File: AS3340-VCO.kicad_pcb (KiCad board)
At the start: 2 copper layers, 90.9 x 101.6 mm, 61 parts, among them J1 1V/OCT_INPUT, J10 SAWTOOTH_OUT, J11 TRIANGLE_OUT, J2 1V/OCT_OUT, J3 CV2_INPUT, J4 EXT_PWM_CTRL_INPUT, J5 POSITIVE_HARD_SYNC_INPUT, J6 NEGATIVE_HARD_SYNC_INPUT, J7 SOFT_SYNC_INPUT, J8 FM_INPUT, J9 SQUARE_OUT, SW1 SW_SPDT, U1 TL074, U2 AS3340

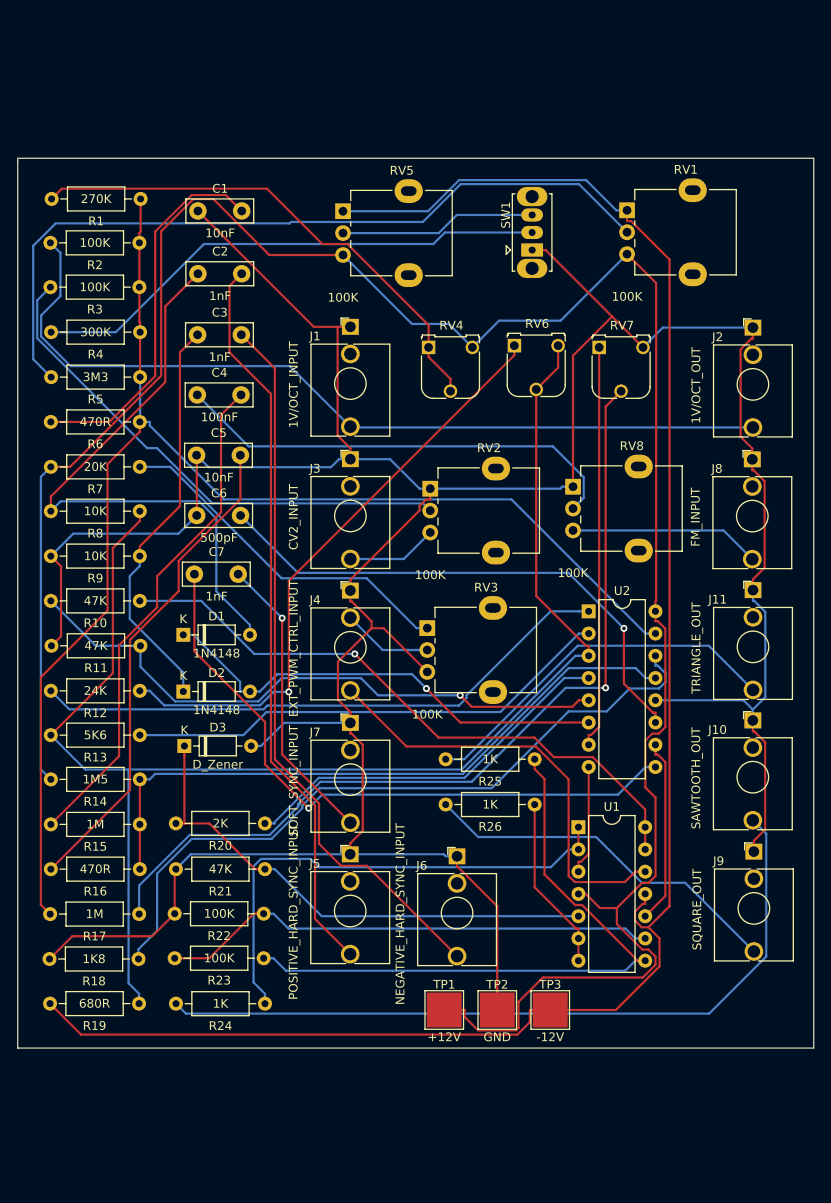
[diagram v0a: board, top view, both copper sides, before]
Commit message: Refactor
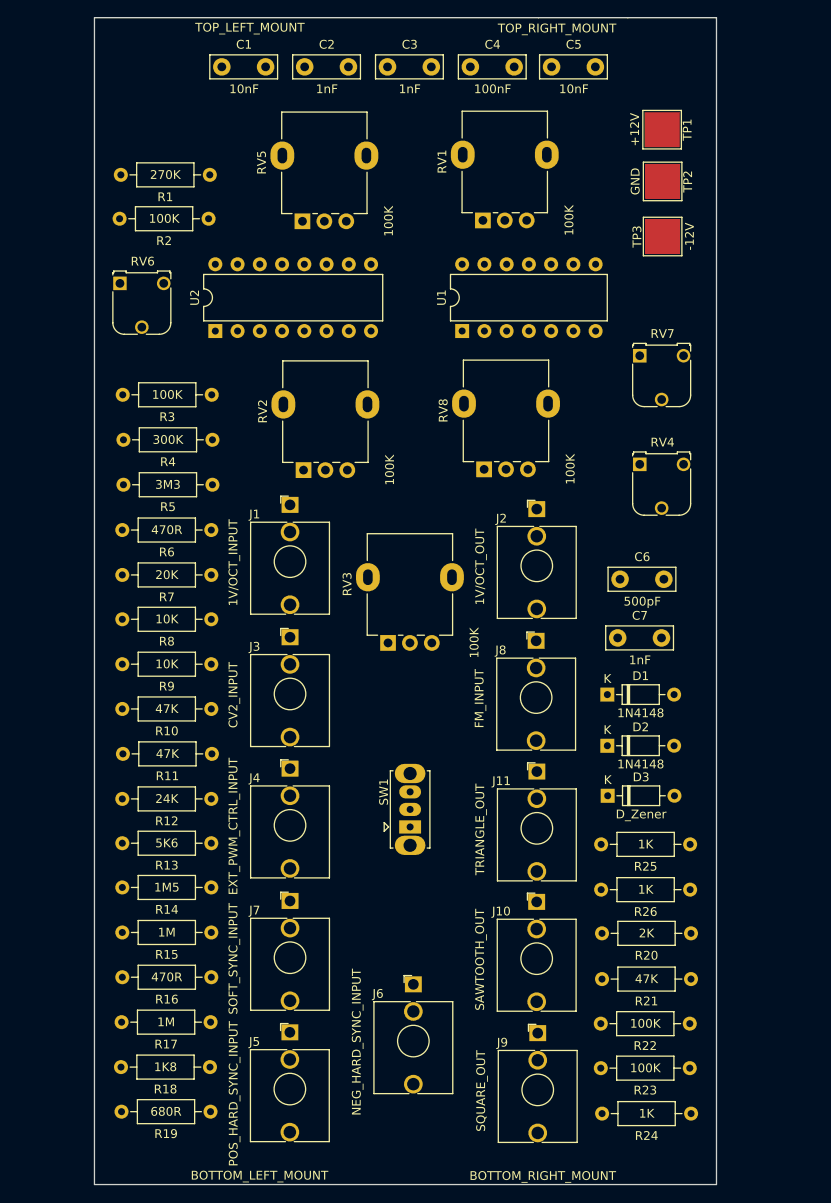
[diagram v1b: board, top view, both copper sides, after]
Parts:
- added BOTTOM_LEFT_MOUNT: MountingHole_3.2mm_M3_Oval, Seattle_Synths:MountingHole_3.2mm_M3_Oval, F.Cu at (115.9, 154.2)
- added BOTTOM_RIGHT_MOUNT: MountingHole_3.2mm_M3_Oval, Seattle_Synths:MountingHole_3.2mm_M3_Oval, F.Cu at (172.1, 154.2)
- added TOP_LEFT_MOUNT: MountingHole_3.2mm_M3_Oval, Seattle_Synths:MountingHole_3.2mm_M3_Oval, F.Cu at (116.0, 27.0)
- added TOP_RIGHT_MOUNT: MountingHole_3.2mm_M3_Oval, Seattle_Synths:MountingHole_3.2mm_M3_Oval, F.Cu at (172.1, 27.0)
- J5: value POSITIVE_HARD_SYNC_INPUT -> POS_HARD_SYNC_INPUT
- J6: value NEGATIVE_HARD_SYNC_INPUT -> NEG_HARD_SYNC_INPUT
- moved TP1 103.5 mm to (173.3, 36.8), turned to 270 degrees
- moved TP2 96.5 mm to (173.4, 42.7), turned to 270 degrees
- moved TP3 89.2 mm to (173.4, 49.0), turned to 90 degrees
- moved SW1 67.3 mm to (144.6, 116.4)
- moved C5 60.1 mm to (160.7, 29.6)
- moved U1 58.2 mm to (150.5, 59.8), turned to 90 degrees
- moved U2 53.3 mm to (122.3, 59.8), turned to 90 degrees
- moved R24 50.2 mm to (166.5, 149.2)
- moved R20 50.2 mm to (166.5, 128.6)
- moved R21 50.2 mm to (166.5, 133.8)
- moved R22 50.2 mm to (166.3, 138.9)
- moved R23 50.2 mm to (166.3, 144.0)
- moved D1 48.9 mm to (167.1, 101.3)
- moved C6 48.9 mm to (168.6, 88.1)
- moved C7 48.9 mm to (168.3, 94.8)
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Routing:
- net GND: track 394.2 -> 0.00 mm
- net +12V: track 261.1 -> 0.00 mm
- net -12V: track 206.1 -> 0.00 mm
- net Net-(R13-Pad1): track 164.5 -> 0.00 mm
- net /FREQ_CTRL: track 156.2 -> 0.00 mm
- net Net-(R17-Pad2): track 100.6 -> 0.00 mm, vias 1 -> 0
- net Net-(J1-PadT): track 97.7 -> 0.00 mm
- net Net-(R5-Pad1): track 88.8 -> 0.00 mm
- net /SAWTOOTH_OUT: track 86.8 -> 0.00 mm
- net Net-(C2-Pad2): track 84.0 -> 0.00 mm
- net Net-(C3-Pad2): track 82.9 -> 0.00 mm
- net Net-(R18-Pad2): track 81.5 -> 0.00 mm
- net /LINEAR_FM: track 74.9 -> 0.00 mm
- net Net-(R23-Pad2): track 74.0 -> 0.00 mm
- net /SOFT_SYNC: track 73.7 -> 0.00 mm, vias 1 -> 0
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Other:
- board size 90.9 x 101.6 mm -> 71 x 133.2 mm
